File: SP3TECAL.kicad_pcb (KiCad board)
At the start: 2 copper layers, 50.8 x 50.8 mm, 22 parts, among them IC1 MM5230-03NDB-TR, IC2 MM5230-03NDB-TR, IC3 MM5230-03NDB-TR, IC4 MM5230-03NDB-TR, J1 Conn_Coaxial, J2 Conn_Coaxial, J3 Conn_Coaxial, J4 Conn_Coaxial, J5 Conn_01x04, J6 Conn_01x04, J7 Conn_01x02, J8 Conn_01x06

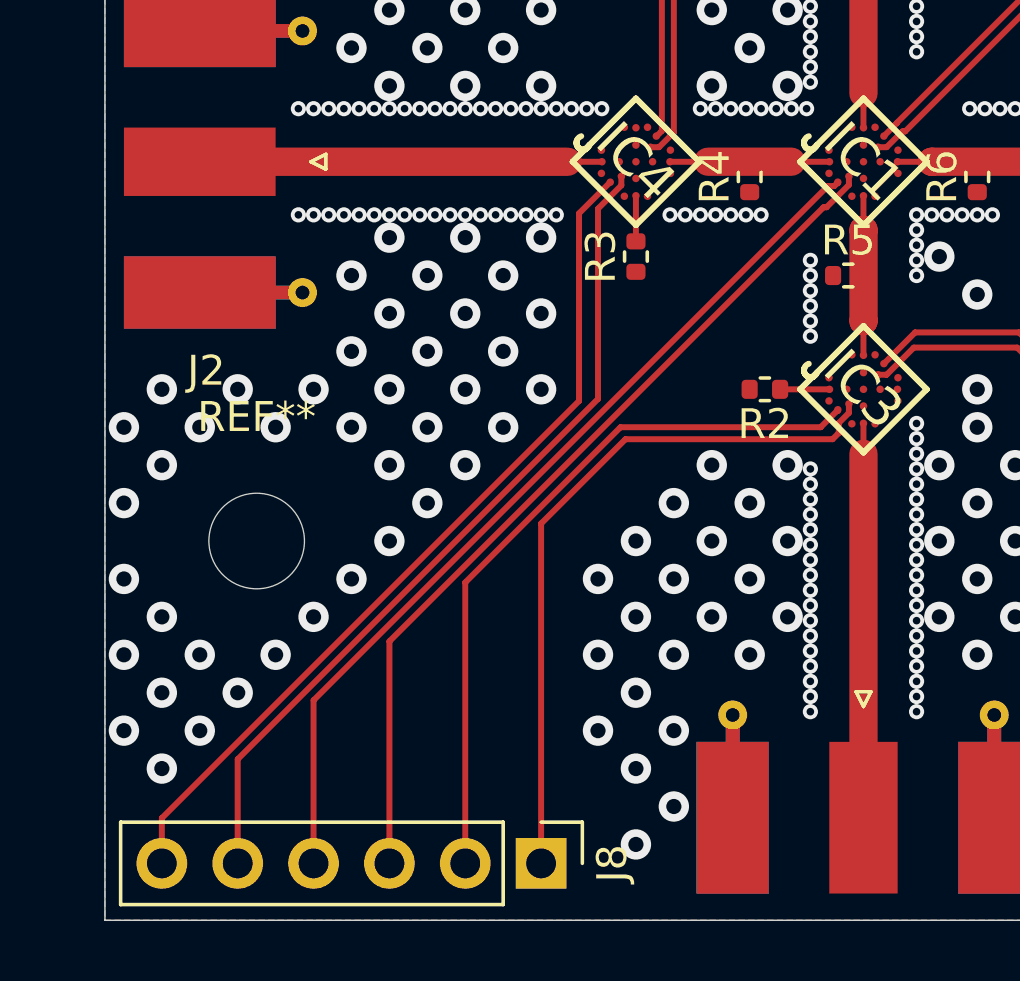
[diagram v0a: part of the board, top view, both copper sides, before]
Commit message: made a southwest microwave launch and put it in the thru
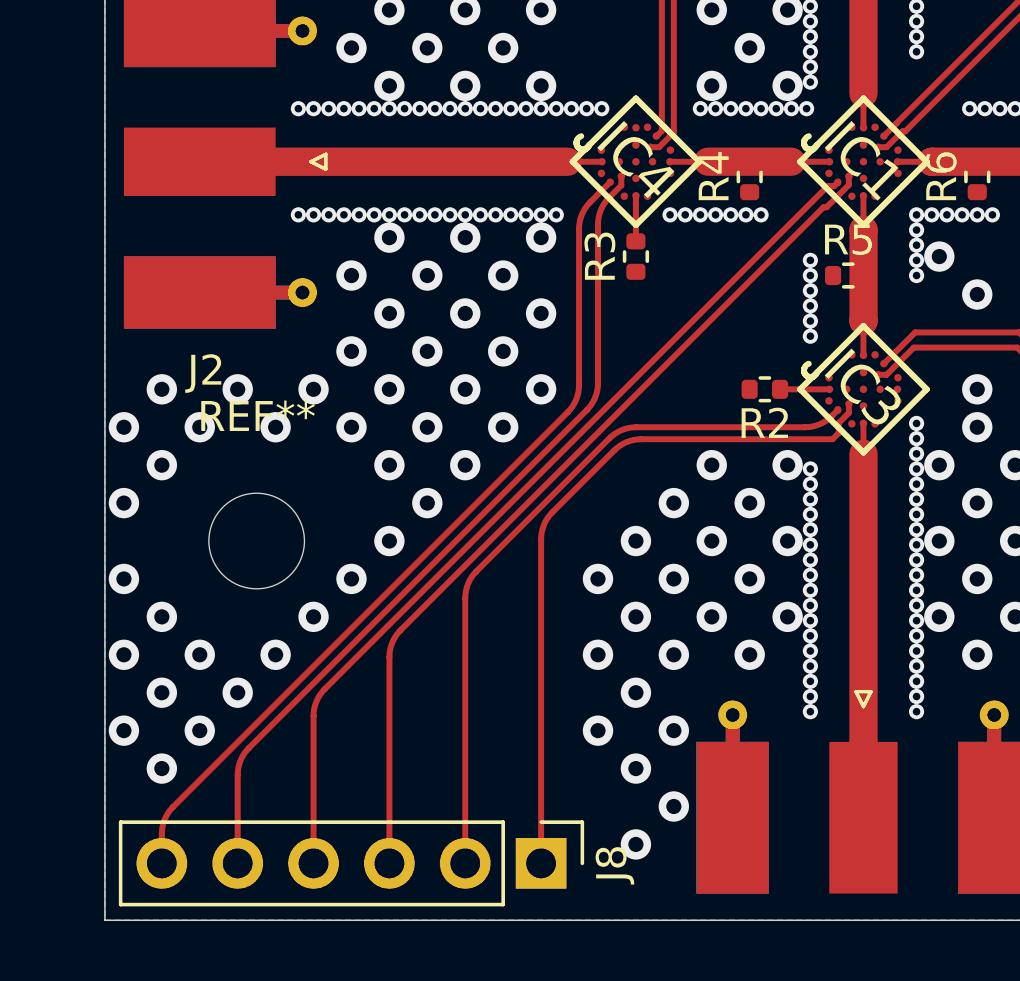
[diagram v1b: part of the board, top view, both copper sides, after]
